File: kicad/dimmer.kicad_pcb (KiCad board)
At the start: 2 copper layers, 60 x 60 mm, 29 parts, among them J1 FTDI, J2 AC IN, J3 Load Out, J4 LED_BYPASS, Q1 S8550 PNP, SW1 Reset, SW2 Prog, T1 Myrra_47121, U1 ESP-03, U2 MOC3021M, U3 4N25

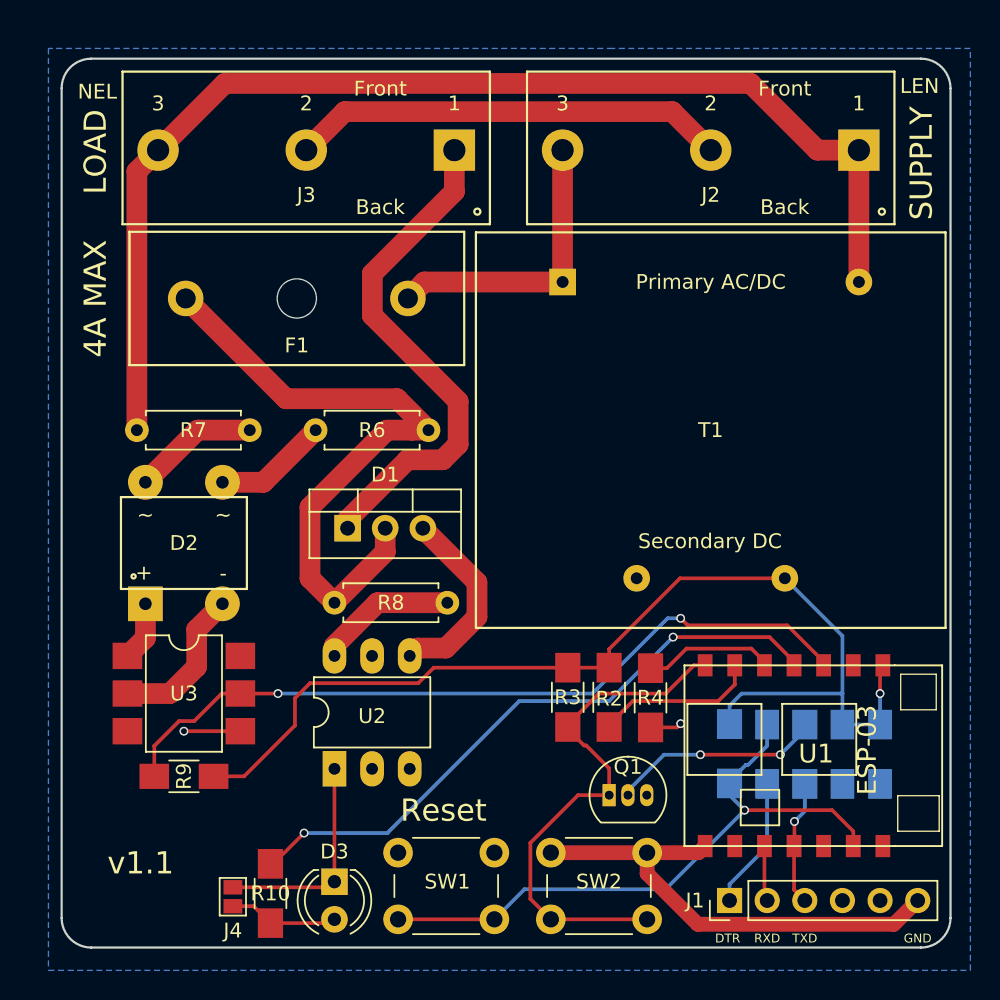
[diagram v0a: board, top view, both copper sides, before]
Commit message: Update for v1.2 - Fixes and board redesign
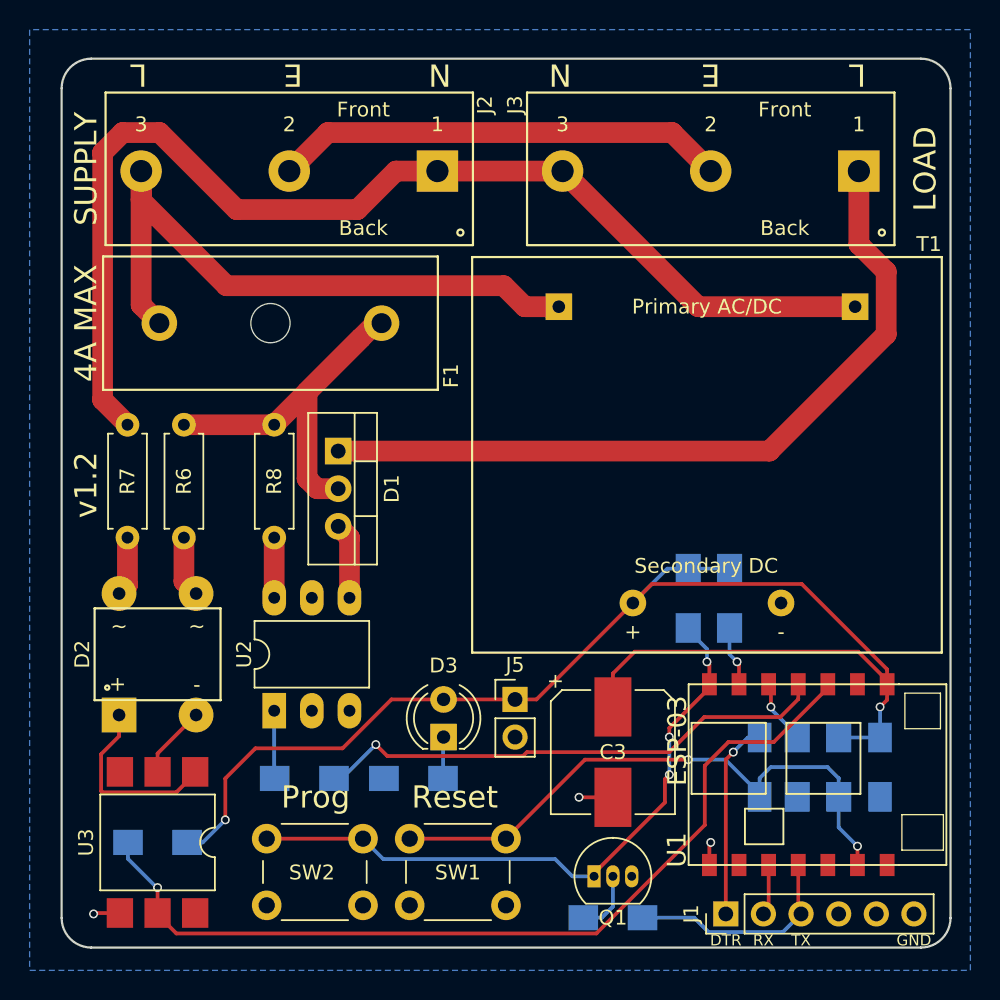
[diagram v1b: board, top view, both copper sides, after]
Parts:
- removed G***: LOGO, tmp:Hello_Kitty
- removed J4: LED_BYPASS, Connectors:GS2
- added J5: PWRIN, Pin_Headers:Pin_Header_Straight_1x02_Pitch2.54mm, F.Cu at (149.6, 111.3)
- added R11: 330, Resistors_SMD:R_1206_HandSoldering, B.Cu at (142.7, 116.6)
- C3: footprint Capacitors_SMD:C_1206_HandSoldering -> Capacitors_SMD:CP_Elec_8x10.5; moved to F.Cu
- D1: footprint TO_SOT_Packages_THT:TO-220_Vertical -> TO_SOT_Packages_THT:TO-220-3_Vertical
- R10, R2, R3, R4, R9: moved to B.Cu
- U3: footprint Housings_DIP:DIP-6_W7.62mm_SMD -> Housings_DIP:SMDIP-6_W9.53mm
- moved J2 28.5 mm to (134.4, 75.4)
- moved J3 27.3 mm to (162.8, 75.4)
- moved C3 18.0 mm to (156.2, 114.8)
- moved R5 17.0 mm to (156.2, 126.0), turned to 180 degrees
- moved SW2 13.2 mm to (139.3, 125.2), turned to 180 degrees
- moved R8 12.5 mm to (133.3, 100.3), turned to 90 degrees
- moved D3 12.2 mm to (144.8, 113.8), turned to 90 degrees
- moved R6 11.5 mm to (127.3, 100.3), turned to 90 degrees
- moved R7 11.0 mm to (123.4, 100.3), turned to 90 degrees
- moved R4 11.0 mm to (168.7, 115.8)
- moved R2 10.5 mm to (164.1, 104.4)
- moved R3 10.5 mm to (161.3, 104.4)
- moved U3 10.2 mm to (125.5, 120.9), turned to 270 degrees
- moved SW1 8.11 mm to (149.0, 125.2), turned to 180 degrees
- moved R10 8.09 mm to (135.4, 116.6), turned to 180 degrees
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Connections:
- D3 pad 2: Net-(D3-Pad2) -> +3V3
- R10 pad 2: Net-(D3-Pad2) -> Net-(R10-Pad2)
- T1 pad 1: /esp8266-base/AC+ -> /esp8266-base/AC-
- T1 pad 5: /esp8266-base/AC- -> /esp8266-base/AC+
- U2 pad 1: Net-(D3-Pad1) -> Net-(R10-Pad2)
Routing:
- net GND: track 38.3 -> 5.65 mm, vias 2 -> 3
- net /esp8266-base/AC+: track 19.8 -> 43.9 mm
- net +3V3: track 73.4 -> 96.0 mm, vias 1 -> 2
- net /DimmedLiveOut: track 34.7 -> 52.0 mm
- net Net-(D1-Pad2): track 43.9 -> 29.5 mm
- net Net-(D3-Pad1): track 14.6 -> 2.81 mm
- net Net-(Q1-Pad2): track 14.3 -> 4.36 mm, vias 2 -> 0
- net /ZeroCrossingOut: track 52.3 -> 61.0 mm, vias 2 -> 1
- net Net-(D2-Pad1): track 4.02 -> 12.7 mm
- net Net-(D1-Pad3): track 13.1 -> 5.14 mm
- net /esp8266-base/GPIO0: track 35.8 -> 43.7 mm, vias 0 -> 3
- net /DimmerIn: track 42.8 -> 35.2 mm, vias 2 -> 1
- net Net-(D3-Pad2): track 7.43 -> 0.00 mm
- net Net-(R2-Pad2): track 11.1 -> 4.07 mm, vias 0 -> 1
- net /esp8266-base/TXD: track 8.48 -> 15.0 mm, vias 1 -> 0
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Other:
- board text added: "Prog"
- board text added: "RX"
- board text added: "TX"
- board text added: "kiall.macinnes.ie/p/esp8266-dimmer v1.2"
- board text added: "v1.2"
- board text removed: "LEN"
- board text removed: "NEL"
- board text removed: "RXD"
- board text removed: "TXD"
- board text removed: "kiall.macinnes.ie/p/esp8266-dimmer v1.1"
- board text removed: "v1.1"
